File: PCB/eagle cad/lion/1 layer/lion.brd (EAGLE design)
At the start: 83.8 x 54 mm, 23 parts, among them IC1 PIC18F4550_40

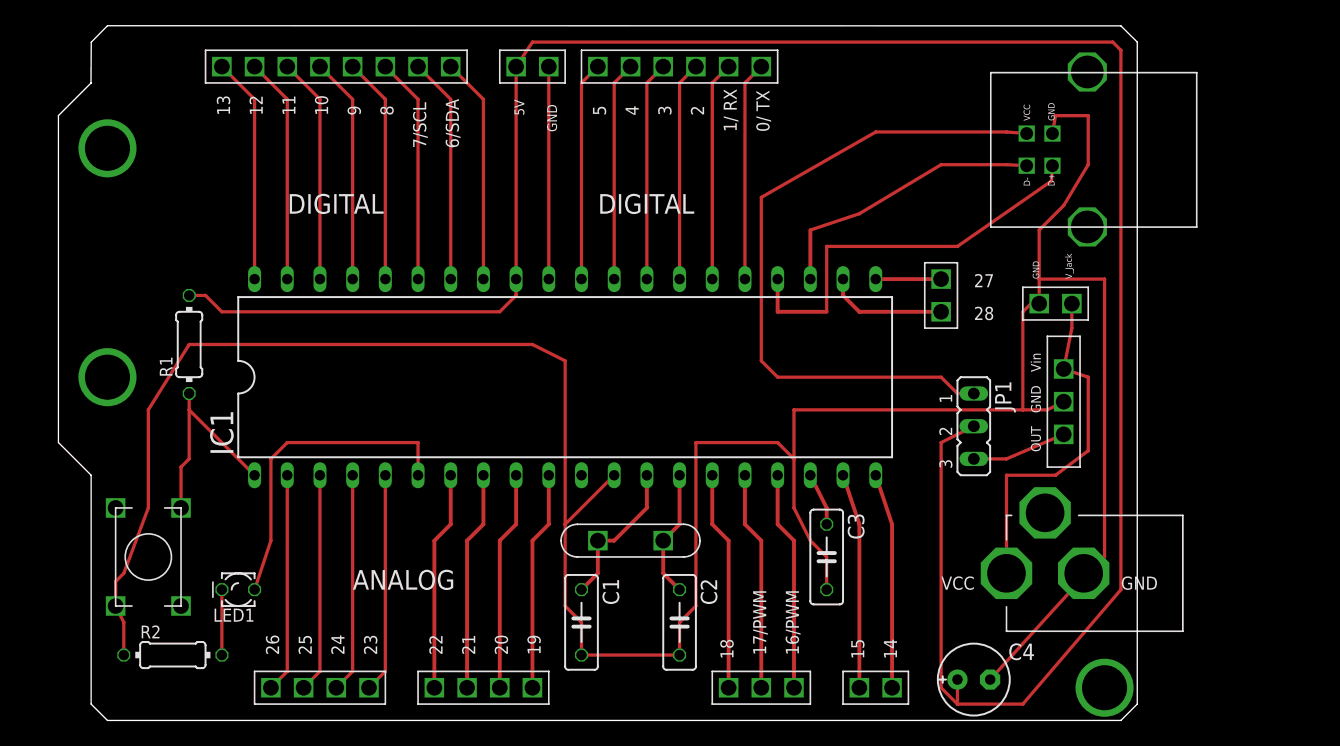
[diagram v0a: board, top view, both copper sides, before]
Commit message: PCB updated
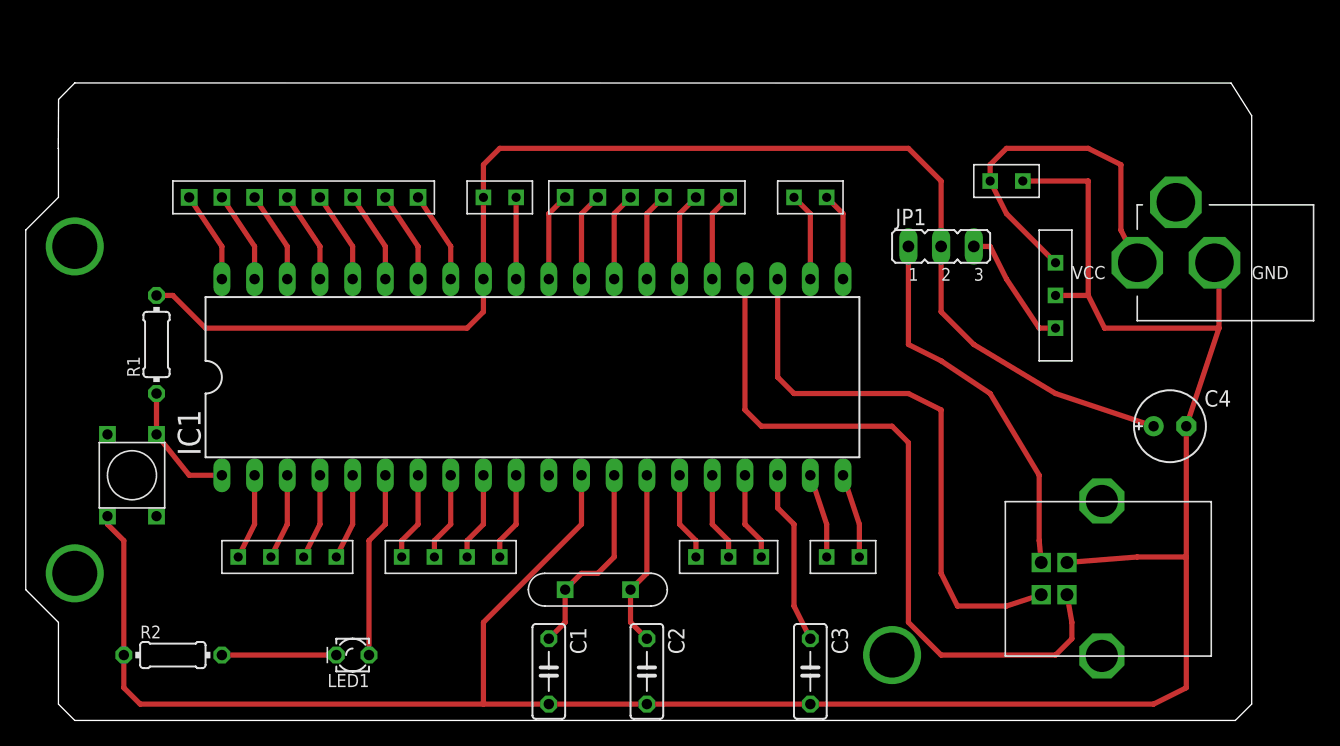
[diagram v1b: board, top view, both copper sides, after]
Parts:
- moved U$1 33.3 mm to (81.1, 5.00)
- moved JACK9V 26.2 mm to (83.8, 35.6)
- moved C4 24.9 mm to (86.4, 22.9)
- moved JP1 14.2 mm to (68.6, 36.8), turned to 0 degrees
- moved U$8 10.9 mm to (59.7, 40.6), turned to 180 degrees
- moved BUTTON1 10.9 mm to (5.71, 19.1)
- moved U$10 10.5 mm to (26.7, 12.7)
- moved U$3 10.5 mm to (49.5, 12.7)
- moved U$6 10.5 mm to (59.7, 12.7)
- moved U$9 10.5 mm to (14.0, 12.7)
- moved U$4 10.5 mm to (52.1, 40.6)
- moved U$5 10.5 mm to (27.9, 40.6)
- moved U$7 10.5 mm to (35.6, 40.6)
- moved LED1 10.2 mm to (22.9, 5.08)
- moved U$12 9.61 mm to (74.9, 41.9), turned to 180 degrees
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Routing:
- net N$30: track 176.8 -> 104.7 mm
- net GND: track 223.2 -> 189.2 mm
- net N$3: track 31.7 -> 55.6 mm
- net +5V: track 52.2 -> 29.2 mm
- net N$8: track 21.9 -> 43.3 mm
- net N$26: track 17.6 -> 7.12 mm
- net N$24: track 17.6 -> 7.12 mm
- net N$25: track 17.6 -> 7.12 mm
- net N$23: track 17.6 -> 7.12 mm
- net N$22: track 17.6 -> 7.12 mm
- net N$21: track 17.6 -> 7.12 mm
- net N$20: track 17.6 -> 7.12 mm
- net N$19: track 17.6 -> 7.12 mm
- net N$14: track 17.0 -> 6.65 mm
- net N$12: track 17.0 -> 6.65 mm
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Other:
- board size 83.8 x 54 mm -> 95.2 x 49.5 mm
- board text added: "D0"
- board text added: "D0/SDA"
- board text added: "D1/SCL"
- board text added: "D2"
- board text added: "D3"
- board text added: "D4"
- board text added: "D5"
- board text added: "D6"
- board text added: "D7"
- board text removed: "0/ TX"
- board text removed: "1/ RX"
- board text removed: "10"
- board text removed: "11"
- board text removed: "12"
- board text removed: "13"
- board text removed: "14"
- board text removed: "15"
- board text removed: "16/PWM"
- board text removed: "17/PWM"
- board text removed: "18"
- board text removed: "19"
- board text removed: "2"
- board text removed: "20"
- board text removed: "21"
- board text removed: "22"
- board text removed: "23"
- board text removed: "24"
- board text removed: "25"
- board text removed: "26"
- board text removed: "27"
- board text removed: "28"
- board text removed: "3"
- board text removed: "4"
- board text removed: "5"
- board text removed: "6/SDA"
- board text removed: "7/SCL"
- board text removed: "8"
- board text removed: "9"
- board text removed: "ANALOG"
- board text removed: "DIGITAL"
- board text removed: "V_Jack"
